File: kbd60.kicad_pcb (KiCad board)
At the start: 2 copper layers, 290 x 100 mm, 164 parts, among them J1 5077CR-16-SMC2-BK-TR, SW1 ESC, SW10 9, SW11 0, SW12 -, SW13 =, SW14 Backspace, SW15 Tab, SW16 Q, SW17 W, SW18 E, SW19 R, SW2 1, SW20 T, SW21 Y, SW22 U, SW23 I, SW24 O, SW25 P, SW26 [, SW27 ], SW28 \, SW29 CapsLock, SW3 2, SW30 A, SW31 S, SW32 D, SW33 F, SW34 G, SW35 H, SW36 J, SW37 K, SW38 L, SW39 ;, SW4 3, SW40 ', SW41 Enter, SW42 ShiftL, SW43 Z, SW44 X, SW45 C, SW46 V, SW47 B, SW48 N, SW49 M, SW5 4, SW50 ,, SW51 ., SW52 /, SW53 ShiftR, SW54 CtrlL, SW55 SuperL, SW56 AltL, SW57 Space, SW58 Fn, SW59 SuperR, SW6 5, SW60 AltR, SW61 CtrlR, SW7 6, SW8 7, SW9 8, U1 RP2040, U2 NJM12877F33, U3 W25Q16JVUXIQ, Y1 FA238V

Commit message: wip: pcb routed
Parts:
- D63, D64, D65, D66, R5, R6, R7, R8: moved to F.Cu
- moved R5 0.30 mm to (319.1, 135.2)
- moved R6 0.30 mm to (319.1, 137.2)
- moved R8 0.30 mm to (319.1, 141.2)
- moved D63 0.29 mm to (321.6, 135.2)
- moved D64 0.29 mm to (321.6, 137.2)
- moved D65 0.29 mm to (321.6, 139.2)
- moved D66 0.29 mm to (321.6, 141.2)
- moved R7 0.29 mm to (319.1, 139.2)
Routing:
- net GND: track 32.9 -> 114.0 mm, vias 11 -> 13
- net Net-(D65-A): track 0.00 -> 1.21 mm
- net Net-(D66-A): track 0.00 -> 1.20 mm
- net Net-(D64-A): track 0.00 -> 1.20 mm
- net Net-(D63-A): track 0.00 -> 1.20 mm
- net /LED4: track 23.3 -> 23.6 mm, vias 0 -> 1
- net /LED2: track 24.6 -> 24.9 mm, vias 0 -> 1
- net /LED1: track 25.3 -> 25.6 mm, vias 0 -> 1
- net /LED3: track 24.0 -> 24.2 mm, vias 0 -> 1

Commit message: wip: re-route columns
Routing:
- net /COL13: track 131.4 -> 122.1 mm
- net /COL10: track 176.2 -> 171.2 mm
- net /COL11: track 156.0 -> 151.3 mm
- net /COL6: track 241.8 -> 237.1 mm
- net /COL2: track 349.4 -> 345.1 mm
- net /COL5: track 241.9 -> 237.9 mm
- net /COL9: track 163.3 -> 159.4 mm
- net /COL8: track 182.6 -> 178.6 mm
- net /COL7: track 202.2 -> 198.3 mm
- net /COL4: track 280.9 -> 276.9 mm
- net /COL1: track 362.5 -> 358.7 mm
- net /COL3: track 324.8 -> 321.3 mm
- net /COL12: track 93.2 -> 90.6 mm
- net /COL14: track 86.1 -> 84.2 mm

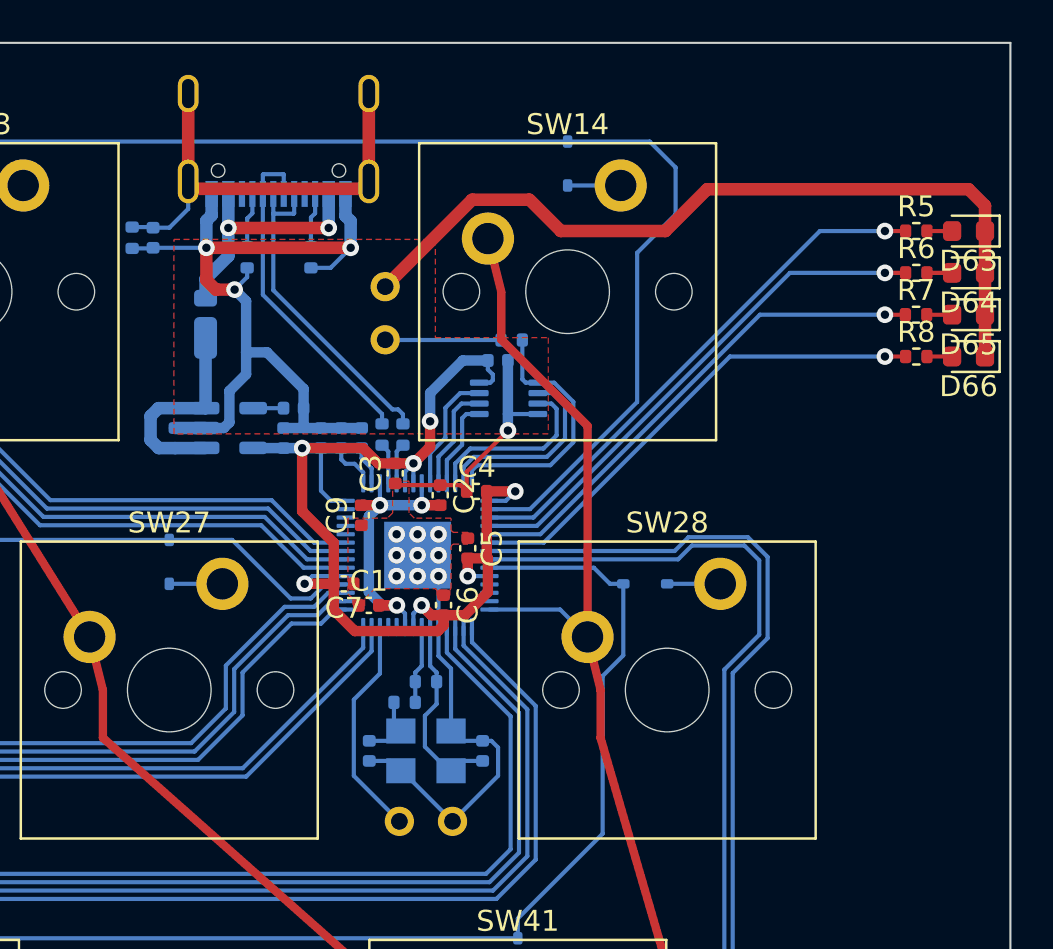
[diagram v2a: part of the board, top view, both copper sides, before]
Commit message: wip: update F.Cu
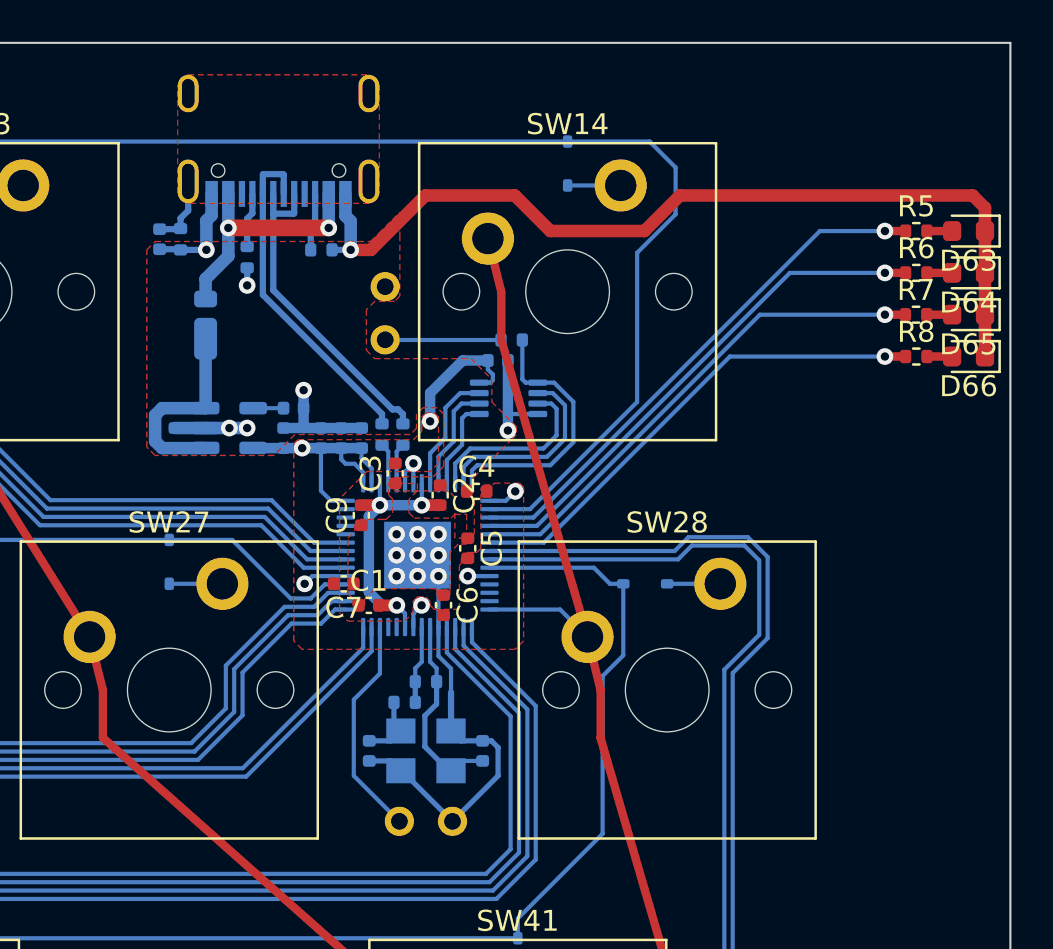
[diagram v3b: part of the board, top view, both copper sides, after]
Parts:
- moved R12 2.32 mm to (283.9, 135.6)
- moved R4 0.61 mm to (290.6, 136.1), turned to 0 degrees
- moved C18 0.32 mm to (282.9, 135.6)
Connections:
- net Net-(J1-SHIELD) renamed /SHIELD
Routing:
- net +3V3: track 63.0 -> 27.2 mm
- net GND: track 114.0 -> 85.0 mm, vias 13 -> 16
- net /SHIELD: track 21.7 -> 3.42 mm
- net /COL14: track 84.2 -> 83.0 mm
- added copper zone on F.Cu, net +3V3
- added copper zone on F.Cu, net /SHIELD

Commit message: wip: update footprint libs
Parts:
- SW1, SW10, SW11, SW12, SW13, SW16, SW17, SW18, SW19, SW2, SW20, SW21, SW22, SW23, SW24, SW25, SW26, SW27, SW3, SW30, SW31, SW32, SW33, SW34, SW35, SW36, SW37, SW38, SW39, SW4, SW40, SW43, SW44, SW45, SW46, SW47, SW48, SW49, SW5, SW50, SW51, SW52, SW6, SW7, SW8, SW9: footprint PCM_Switch_Keyboard_Cherry_MX:SW_Cherry_MX_PCB_1.00u -> Button_Switch_Keyboard:SW_Cherry_MX_1.00u_PCB
- SW14: footprint PCM_Switch_Keyboard_Cherry_MX:SW_Cherry_MX_PCB_2.00u -> Button_Switch_Keyboard:SW_Cherry_MX_2.00u_PCB
- SW15, SW28: footprint PCM_Switch_Keyboard_Cherry_MX:SW_Cherry_MX_PCB_1.50u -> Button_Switch_Keyboard:SW_Cherry_MX_1.50u_PCB
- SW29: footprint PCM_Switch_Keyboard_Cherry_MX:SW_Cherry_MX_PCB_1.75u -> Button_Switch_Keyboard:SW_Cherry_MX_1.75u_PCB
- SW41, SW42: footprint PCM_Switch_Keyboard_Cherry_MX:SW_Cherry_MX_PCB_2.25u -> Button_Switch_Keyboard:SW_Cherry_MX_2.25u_PCB
- SW53: footprint PCM_Switch_Keyboard_Cherry_MX:SW_Cherry_MX_PCB_2.75u -> Button_Switch_Keyboard:SW_Cherry_MX_2.75u_PCB
- SW54, SW55, SW56, SW58, SW59, SW60, SW61: footprint PCM_Switch_Keyboard_Cherry_MX:SW_Cherry_MX_PCB_1.25u -> Button_Switch_Keyboard:SW_Cherry_MX_1.25u_PCB
- SW57: footprint PCM_Switch_Keyboard_Cherry_MX:SW_Cherry_MX_PCB_6.25u -> Button_Switch_Keyboard:SW_Cherry_MX_6.25u_PCB
- moved SW12 5.68 mm to (257.3, 133.0)
- moved SW13 5.68 mm to (276.4, 133.0)
- moved SW14 5.68 mm to (305.0, 133.0)
- moved SW33 5.68 mm to (138.3, 171.1)
- moved SW38 5.68 mm to (233.5, 171.1)
- moved SW59 5.68 mm to (264.5, 209.2)
- moved SW60 5.68 mm to (288.3, 209.2)
- moved SW61 5.68 mm to (312.1, 209.2)
- moved SW7 5.68 mm to (162.1, 133.0)
- moved SW3 5.68 mm to (85.9, 133.0)
- moved SW30 5.68 mm to (81.1, 171.1)
- moved SW31 5.68 mm to (100.2, 171.1)
- moved SW4 5.68 mm to (104.9, 133.0)
- moved SW5 5.68 mm to (124.0, 133.0)
- moved SW55 5.68 mm to (74.0, 209.2)
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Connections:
- SW1 pad 1: /COL1 -> Net-(D1-A)
- SW1 pad 2: Net-(D1-A) -> /COL1
- SW10 pad 1: /COL10 -> Net-(D10-A)
- SW10 pad 2: Net-(D10-A) -> /COL10
- SW11 pad 1: /COL11 -> Net-(D11-A)
- SW11 pad 2: Net-(D11-A) -> /COL11
- SW12 pad 1: /COL12 -> Net-(D12-A)
- SW12 pad 2: Net-(D12-A) -> /COL12
- SW13 pad 1: /COL13 -> Net-(D13-A)
- SW13 pad 2: Net-(D13-A) -> /COL13
- SW14 pad 1: /COL14 -> Net-(D14-A)
- SW14 pad 2: Net-(D14-A) -> /COL14
- SW15 pad 1: /COL1 -> Net-(D15-A)
- SW15 pad 2: Net-(D15-A) -> /COL1
- SW16 pad 1: /COL2 -> Net-(D16-A)
- SW16 pad 2: Net-(D16-A) -> /COL2
- SW17 pad 1: /COL3 -> Net-(D17-A)
- SW17 pad 2: Net-(D17-A) -> /COL3
- SW18 pad 1: /COL4 -> Net-(D18-A)
- SW18 pad 2: Net-(D18-A) -> /COL4
- SW19 pad 1: /COL5 -> Net-(D19-A)
- SW19 pad 2: Net-(D19-A) -> /COL5
- SW2 pad 1: /COL2 -> Net-(D2-A)
- SW2 pad 2: Net-(D2-A) -> /COL2
- SW20 pad 1: /COL6 -> Net-(D20-A)
- SW20 pad 2: Net-(D20-A) -> /COL6
- SW21 pad 1: /COL7 -> Net-(D21-A)
- SW21 pad 2: Net-(D21-A) -> /COL7
- SW22 pad 1: /COL8 -> Net-(D22-A)
- SW22 pad 2: Net-(D22-A) -> /COL8
- SW23 pad 1: /COL9 -> Net-(D23-A)
- SW23 pad 2: Net-(D23-A) -> /COL9
- SW24 pad 1: /COL10 -> Net-(D24-A)
- SW24 pad 2: Net-(D24-A) -> /COL10
- SW25 pad 1: /COL11 -> Net-(D25-A)
- SW25 pad 2: Net-(D25-A) -> /COL11
- SW26 pad 1: /COL12 -> Net-(D26-A)
- SW26 pad 2: Net-(D26-A) -> /COL12
- SW27 pad 1: /COL13 -> Net-(D27-A)
- SW27 pad 2: Net-(D27-A) -> /COL13
- SW28 pad 1: /COL14 -> Net-(D28-A)
- SW28 pad 2: Net-(D28-A) -> /COL14
- SW29 pad 1: /COL1 -> Net-(D29-A)
- SW29 pad 2: Net-(D29-A) -> /COL1
- SW3 pad 1: /COL3 -> Net-(D3-A)
- SW3 pad 2: Net-(D3-A) -> /COL3
- SW30 pad 1: /COL2 -> Net-(D30-A)
- SW30 pad 2: Net-(D30-A) -> /COL2
- SW31 pad 1: /COL3 -> Net-(D31-A)
- SW31 pad 2: Net-(D31-A) -> /COL3
- SW32 pad 1: /COL4 -> Net-(D32-A)
- SW32 pad 2: Net-(D32-A) -> /COL4
- SW33 pad 1: /COL5 -> Net-(D33-A)
- SW33 pad 2: Net-(D33-A) -> /COL5
- SW34 pad 1: /COL6 -> Net-(D34-A)
- SW34 pad 2: Net-(D34-A) -> /COL6
- SW35 pad 1: /COL7 -> Net-(D35-A)
- SW35 pad 2: Net-(D35-A) -> /COL7
- SW36 pad 1: /COL8 -> Net-(D36-A)
- SW36 pad 2: Net-(D36-A) -> /COL8
- SW37 pad 1: /COL9 -> Net-(D37-A)
- SW37 pad 2: Net-(D37-A) -> /COL9
- SW38 pad 1: /COL10 -> Net-(D38-A)
- SW38 pad 2: Net-(D38-A) -> /COL10
- SW39 pad 1: /COL11 -> Net-(D39-A)
- SW39 pad 2: Net-(D39-A) -> /COL11
- SW4 pad 1: /COL4 -> Net-(D4-A)
- SW4 pad 2: Net-(D4-A) -> /COL4
- SW40 pad 1: /COL12 -> Net-(D40-A)
- SW40 pad 2: Net-(D40-A) -> /COL12
- SW41 pad 1: /COL13 -> Net-(D41-A)
- SW41 pad 2: Net-(D41-A) -> /COL13
- SW42 pad 1: /COL1 -> Net-(D42-A)
- SW42 pad 2: Net-(D42-A) -> /COL1
- SW43 pad 1: /COL2 -> Net-(D43-A)
- SW43 pad 2: Net-(D43-A) -> /COL2
- SW44 pad 1: /COL3 -> Net-(D44-A)
- SW44 pad 2: Net-(D44-A) -> /COL3
- SW45 pad 1: /COL4 -> Net-(D45-A)
- SW45 pad 2: Net-(D45-A) -> /COL4
- SW46 pad 1: /COL5 -> Net-(D46-A)
- SW46 pad 2: Net-(D46-A) -> /COL5
- SW47 pad 1: /COL6 -> Net-(D47-A)
- SW47 pad 2: Net-(D47-A) -> /COL6
- SW48 pad 1: /COL7 -> Net-(D48-A)
- SW48 pad 2: Net-(D48-A) -> /COL7
- SW49 pad 1: /COL8 -> Net-(D49-A)
- SW49 pad 2: Net-(D49-A) -> /COL8
- SW5 pad 1: /COL5 -> Net-(D5-A)
- SW5 pad 2: Net-(D5-A) -> /COL5
- SW50 pad 1: /COL9 -> Net-(D50-A)
- SW50 pad 2: Net-(D50-A) -> /COL9
- SW51 pad 1: /COL10 -> Net-(D51-A)
- SW51 pad 2: Net-(D51-A) -> /COL10
- SW52 pad 1: /COL11 -> Net-(D52-A)
- SW52 pad 2: Net-(D52-A) -> /COL11
- SW53 pad 1: /COL13 -> Net-(D53-A)
- SW53 pad 2: Net-(D53-A) -> /COL13
- SW54 pad 1: /COL1 -> Net-(D54-A)
- SW54 pad 2: Net-(D54-A) -> /COL1
- SW55 pad 1: /COL2 -> Net-(D55-A)
- SW55 pad 2: Net-(D55-A) -> /COL2
- SW56 pad 1: /COL3 -> Net-(D56-A)
- SW56 pad 2: Net-(D56-A) -> /COL3
- SW57 pad 1: /COL6 -> Net-(D57-A)
- SW57 pad 2: Net-(D57-A) -> /COL6
- SW58 pad 1: /COL10 -> Net-(D58-A)
- SW58 pad 2: Net-(D58-A) -> /COL10
- SW59 pad 1: /COL11 -> Net-(D59-A)
- SW59 pad 2: Net-(D59-A) -> /COL11
- SW6 pad 1: /COL6 -> Net-(D6-A)
- SW6 pad 2: Net-(D6-A) -> /COL6
- SW60 pad 1: /COL13 -> Net-(D60-A)
- SW60 pad 2: Net-(D60-A) -> /COL13
- SW61 pad 1: /COL14 -> Net-(D61-A)
- SW61 pad 2: Net-(D61-A) -> /COL14
- SW7 pad 1: /COL7 -> Net-(D7-A)
- SW7 pad 2: Net-(D7-A) -> /COL7
- SW8 pad 1: /COL8 -> Net-(D8-A)
- SW8 pad 2: Net-(D8-A) -> /COL8
- SW9 pad 1: /COL9 -> Net-(D9-A)
- SW9 pad 2: Net-(D9-A) -> /COL9
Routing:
- net /COL4: track 276.9 -> 273.0 mm
- net /COL3: track 321.3 -> 318.4 mm
- net /COL2: track 345.1 -> 342.7 mm
- net /LED1: track 25.6 -> 27.6 mm
- net /LED2: track 24.9 -> 26.3 mm
- net /COL8: track 178.6 -> 179.8 mm
- net /COL9: track 159.4 -> 160.4 mm
- net /COL1: track 358.7 -> 357.7 mm
- net /COL7: track 198.3 -> 199.2 mm
- net /ROW5: track 333.2 -> 334.2 mm
- net /COL6: track 237.1 -> 238.0 mm
- net /COL10: track 171.2 -> 170.4 mm
- net /COL5: track 237.9 -> 238.8 mm
- net /LED3: track 24.2 -> 24.9 mm
- net /COL13: track 122.1 -> 121.6 mm

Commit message: DRC ok
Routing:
- net GND: track 85.0 -> 72.7 mm, vias 16 -> 18
- net /RUN: track 10.7 -> 11.6 mm
